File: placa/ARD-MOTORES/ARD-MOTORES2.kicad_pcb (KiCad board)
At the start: 2 copper layers, 68.6 x 53.3 mm, 8 parts, among them J1 Power, J2 Digital/PWM, J3 Analog, J4 Digital/PWM

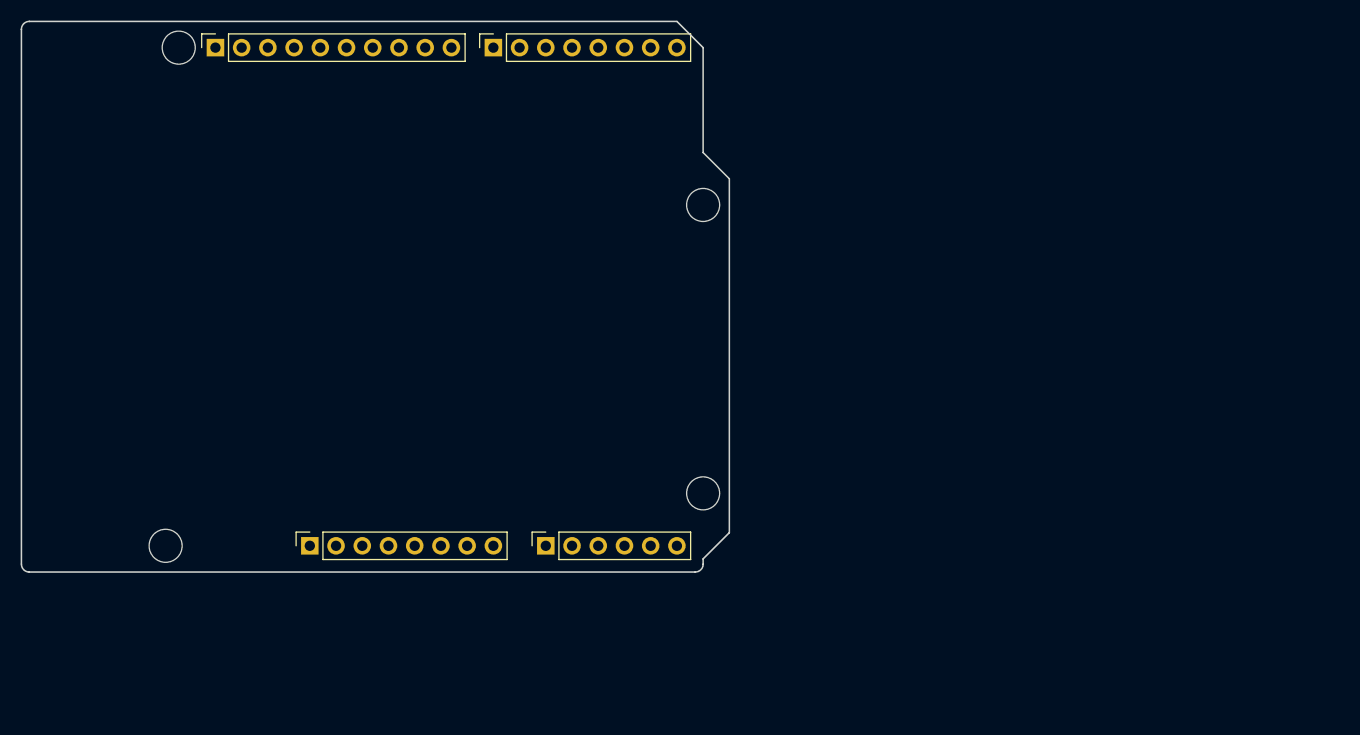
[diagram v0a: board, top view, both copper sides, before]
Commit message: m
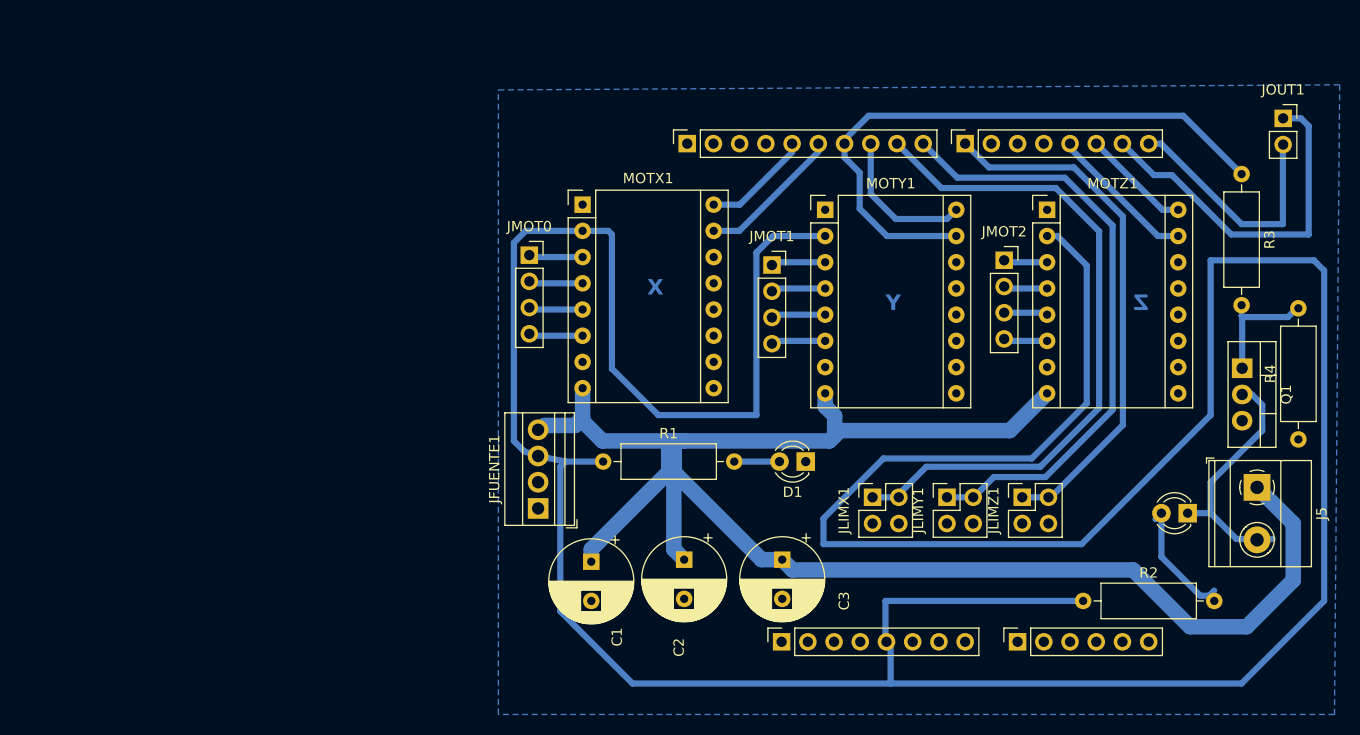
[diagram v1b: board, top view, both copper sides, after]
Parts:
- removed MH1, MH2, MH3, MH4: MountingHole_3.2mm, Arduino_MountingHole:MountingHole_3.2mm
- added C1: C, Capacitor_THT:CP_Radial_D8.0mm_P3.80mm, F.Cu at (155.2, 99.0)
- added C2: C, Capacitor_THT:CP_Radial_D8.0mm_P3.80mm, F.Cu at (164.2, 98.8)
- added C3: C, Capacitor_THT:CP_Radial_D8.0mm_P3.80mm, F.Cu at (173.7, 98.8)
- added D1: LED, LED_THT:LED_D3.0mm, F.Cu at (176.0, 89.3)
- added D4: LED2, LED_THT:LED_D3.0mm, F.Cu at (213.0, 94.3)
- added J5: Conn_01x02, TerminalBlock_Phoenix:TerminalBlock_Phoenix_MKDS-1,5-2-5.08_1x02_P5.08mm_Horizontal, F.Cu at (219.7, 91.8)
- added JFUENTE1: Conn_01x04, TerminalBlock:TerminalBlock_Xinya_XY308-2.54-4P_1x04_P2.54mm_Horizontal, F.Cu at (150.1, 93.8)
- added JLIMX1: 02x02, Connector_PinSocket_2.54mm:PinSocket_2x02_P2.54mm_Vertical, F.Cu at (182.5, 92.8)
- added JLIMY1: 02x02, Connector_PinSocket_2.54mm:PinSocket_2x02_P2.54mm_Vertical, F.Cu at (189.7, 92.8)
- added JLIMZ1: 02x02, Connector_PinSocket_2.54mm:PinSocket_2x02_P2.54mm_Vertical, F.Cu at (197.0, 92.8)
- added JMOT0: Conn_01x04_Pin, Connector_PinSocket_2.54mm:PinSocket_1x04_P2.54mm_Vertical, F.Cu at (149.2, 69.3)
- added JMOT1: Conn_01x04_Pin, Connector_PinSocket_2.54mm:PinSocket_1x04_P2.54mm_Vertical, F.Cu at (172.7, 70.3)
- added JMOT2: Conn_01x04_Pin, Connector_PinSocket_2.54mm:PinSocket_1x04_P2.54mm_Vertical, F.Cu at (195.2, 69.8)
- added JOUT1: Conn_01x02, Connector_PinSocket_2.54mm:PinSocket_1x02_P2.54mm_Vertical, F.Cu at (222.2, 56.0)
- added MOTX1: Pololu_Breakout_A4988, Module:Pololu_Breakout-16_15.2x20.3mm, F.Cu at (154.4, 64.4)
- added MOTY1: Pololu_Breakout_A4988, Module:Pololu_Breakout-16_15.2x20.3mm, F.Cu at (177.9, 64.9)
- added MOTZ1: Pololu_Breakout_A4988, Module:Pololu_Breakout-16_15.2x20.3mm, F.Cu at (199.4, 64.9)
- added Q1: IRLZ44N, Package_TO_SOT_THT:TO-220-3_Vertical, F.Cu at (218.3, 80.3)
- added R1: 330R, Resistor_THT:R_Axial_DIN0309_L9.0mm_D3.2mm_P12.70mm_Horizontal, F.Cu at (156.4, 89.3)
- added R2: 1800R, Resistor_THT:R_Axial_DIN0309_L9.0mm_D3.2mm_P12.70mm_Horizontal, F.Cu at (202.9, 102.8)
- added R3: 10R, Resistor_THT:R_Axial_DIN0309_L9.0mm_D3.2mm_P12.70mm_Horizontal, F.Cu at (218.2, 61.5)
- added R4: 10k, Resistor_THT:R_Axial_DIN0309_L9.0mm_D3.2mm_P12.70mm_Horizontal, F.Cu at (223.7, 87.2)
- moved J1 46.6 mm to (173.6, 106.8)
- moved J4 46.6 mm to (191.4, 58.5)
- moved J2 46.6 mm to (164.5, 58.5)
- moved J3 46.6 mm to (196.5, 106.8)
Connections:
- J1 pad 8: VCC -> unconnected-(J1-Pin_8-Pad8)
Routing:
- net +5V: track 0.00 -> 364.2 mm
- net +12V: track 0.00 -> 169.0 mm
- net /*9: track 0.00 -> 66.2 mm
- net /*11: track 0.00 -> 59.5 mm
- net /8: track 0.00 -> 59.3 mm
- net /7: track 0.00 -> 50.8 mm
- net /TX/1: track 0.00 -> 35.0 mm
- net Net-(D4-K): track 0.00 -> 24.2 mm
- net /RX/0: track 0.00 -> 24.0 mm
- net /*10: track 0.00 -> 14.5 mm
- net /*3: track 0.00 -> 14.4 mm
- net /12: track 0.00 -> 14.1 mm
- net Net-(D4-A): track 0.00 -> 11.9 mm
- net Net-(Q1-G): track 0.00 -> 10.9 mm
- net /2: track 0.00 -> 10.6 mm
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- added copper zone on B.Cu, net GND
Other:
- board outline removed
- board text added: "X"
- board text added: "Y"
- board text added: "Z"
